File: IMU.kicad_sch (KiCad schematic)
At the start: 1 part, among them U2 4754

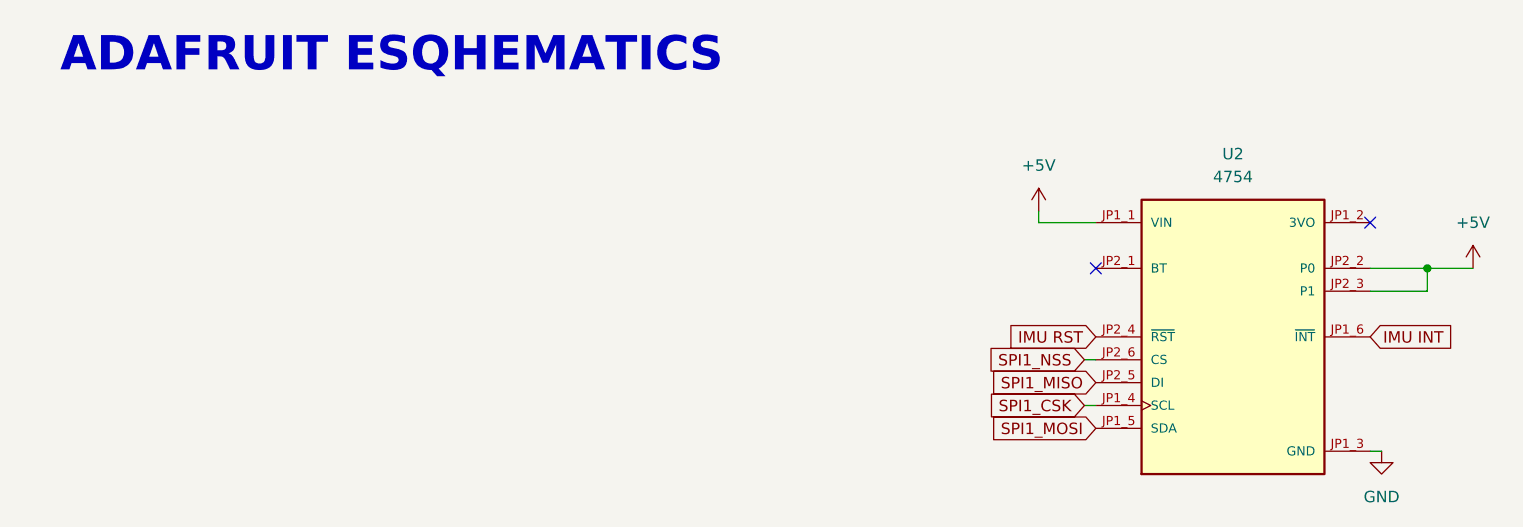
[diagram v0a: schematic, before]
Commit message: Todo antes de PCB
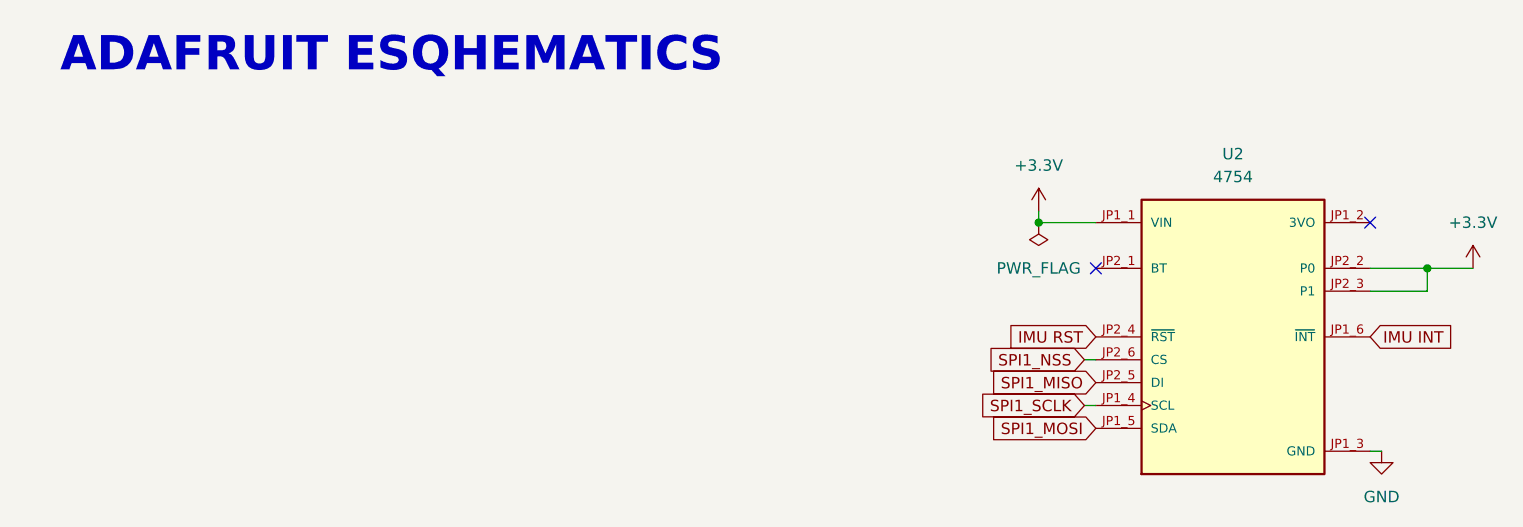
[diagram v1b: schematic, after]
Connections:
- net +5V renamed +3.3V
- net SPI1_CSK renamed SPI1_SCLK
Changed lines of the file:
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@@
 		(color 0 0 0 0)
 	)
+	(junction
+		(at 143.51 95.25)
+		(diameter 0)
+		(color 0 0 0 0)
+	)
 	(no_connect
 		(at 180.34 95.25)
@@
 		)
 	)
-	(global_label "SPI1_CSK"
+	(global_label "SPI1_SCLK"
 		(shape input)
 		(at 148.59 115.57 180)
@@
 		)
 		(property "Intersheetrefs" "${INTERSHEET_REFS}"
-			(at 136.5939 115.57 0)
+			(at 135.5658 115.57 0)
 			(hide yes)
 			(show_name no)
@@
 	)
 	(symbol
-		(lib_id "power:+5V")
-		(at 143.51 93.98 0)
-		(unit 1)
-		(body_style 1)
-		(exclude_from_sim no)
-		(in_bom yes)
-		(on_board yes)
-		(in_pos_files yes)
-		(dnp no)
-		(fields_autoplaced yes)
-		(property "Reference" "#PWR028"
-			(at 143.51 97.79 0)
-			(hide yes)
-			(show_name no)
-			(do_not_autoplace no)
-			(effects
-				(font
-					(size 1.27 1.27)
-				)
-			)
-		)
-		(property "Value" "+5V"
-			(at 143.51 88.9 0)
-			(show_name no)
-			(do_not_autoplace no)
-			(effects
-				(font
-					(size 1.27 1.27)
-				)
-			)
-		)
-		(property "Footprint" ""
-			(at 143.51 93.98 0)
-			(hide yes)
-			(show_name no)
-			(do_not_autoplace no)
-			(effects
-				(font
-					(size 1.27 1.27)
-				)
-			)
-		)
-		(property "Datasheet" ""
-			(at 143.51 93.98 0)
-			(hide yes)
-			(show_name no)
-			(do_not_autoplace no)
-			(effects
-				(font
-					(size 1.27 1.27)
-				)
-			)
-		)
-		(property "Description" "Power symbol creates a global label with name \"+5V\""
-			(at 143.51 93.98 0)
-			(hide yes)
-			(show_name no)
-			(do_not_autoplace no)
-			(effects
-				(font
-					(size 1.27 1.27)
-				)
-			)
-		)
-		(pin "1"
-		)
-		(instances
-			(project "ARLISS_STM32_2026"
-				(path "/9719ea46-14c4-4409-9c57-49dd5454c03f/243e1b39-32df-463e-8f3d-bc06fe39ea80"
-					(reference "#PWR028")
-					(unit 1)
-				)
-			)
-		)
-	)
-	(symbol
 		(lib_id "4754:4754")
 		(at 165.1 107.95 0)
@@
 			(at 165.1 107.95 0)
 			(hide yes)
-			(show_name no)
+			(show_name yes)
 			(do_not_autoplace no)
 			(effects
@@
 	)
 	(symbol
-		(lib_id "power:+5V")
+		(lib_id "power:+3.3V")
+		(at 143.51 93.98 0)
+		(unit 1)
+		(body_style 1)
+		(exclude_from_sim no)
+		(in_bom yes)
+		(on_board yes)
+		(in_pos_files yes)
+		(dnp no)
+		(fields_autoplaced yes)
+		(property "Reference" "#PWR028"
+			(at 143.51 97.79 0)
+			(hide yes)
+			(show_name no)
+			(do_not_autoplace no)
+			(effects
+				(font
+					(size 1.27 1.27)
+				)
+			)
+		)
+		(property "Value" "+3.3V"
+			(at 143.51 88.9 0)
+			(show_name no)
+			(do_not_autoplace no)
+			(effects
+				(font
+					(size 1.27 1.27)
+				)
+			)
+		)
+		(property "Footprint" ""
+			(at 143.51 93.98 0)
+			(hide yes)
+			(show_name no)
+			(do_not_autoplace no)
+			(effects
+				(font
+					(size 1.27 1.27)
+				)
+			)
+		)
+		(property "Datasheet" ""
+			(at 143.51 93.98 0)
+			(hide yes)
+			(show_name no)
+			(do_not_autoplace no)
+			(effects
+				(font
+					(size 1.27 1.27)
+				)
+			)
+		)
+		(property "Description" "Power symbol creates a global label with name \"+3.3V\""
+			(at 143.51 93.98 0)
+			(hide yes)
+			(show_name no)
+			(do_not_autoplace no)
+			(effects
+				(font
+					(size 1.27 1.27)
+				)
+			)
+		)
+		(pin "1"
+		)
+		(instances
+			(project "ARLISS_STM32_2026"
+				(path "/9719ea46-14c4-4409-9c57-49dd5454c03f/243e1b39-32df-463e-8f3d-bc06fe39ea80"
+					(reference "#PWR028")
+					(unit 1)
+				)
+			)
+		)
+	)
+	(symbol
+		(lib_id "power:PWR_FLAG")
+		(at 143.51 95.25 180)
+		(unit 1)
+		(body_style 1)
+		(exclude_from_sim no)
+		(in_bom yes)
+		(on_board yes)
+		(in_pos_files yes)
+		(dnp no)
+		(fields_autoplaced yes)
+		(property "Reference" "#FLG01"
+			(at 143.51 97.155 0)
+			(hide yes)
+			(show_name no)
+			(do_not_autoplace no)
+			(effects
+				(font
+					(size 1.27 1.27)
+				)
+			)
+		)
+		(property "Value" "PWR_FLAG"
+			(at 143.51 100.33 0)
+			(show_name no)
+			(do_not_autoplace no)
+			(effects
+				(font
+					(size 1.27 1.27)
+				)
+			)
+		)
+		(property "Footprint" ""
+			(at 143.51 95.25 0)
+			(hide yes)
+			(show_name no)
+			(do_not_autoplace no)
+			(effects
+				(font
+					(size 1.27 1.27)
+				)
+			)
+		)
+		(property "Datasheet" ""
+			(at 143.51 95.25 0)
+			(hide yes)
+			(show_name no)
+			(do_not_autoplace no)
+			(effects
+				(font
+					(size 1.27 1.27)
+				)
+			)
+		)
+		(property "Description" "Special symbol for telling ERC where power comes from"
+			(at 143.51 95.25 0)
+			(hide yes)
+			(show_name no)
+			(do_not_autoplace no)
+			(effects
+				(font
+					(size 1.27 1.27)
+				)
+			)
+		)
+		(pin "1"
+		)
+		(instances
+			(project "ARLISS_STM32_2026"
+				(path "/9719ea46-14c4-4409-9c57-49dd5454c03f/243e1b39-32df-463e-8f3d-bc06fe39ea80"
+					(reference "#FLG01")
+					(unit 1)
+				)
+			)
+		)
+	)
+	(symbol
+		(lib_id "power:+3.3V")
 		(at 191.77 100.33 0)
 		(unit 1)
@@
 			)
 		)
-		(property "Value" "+5V"
+		(property "Value" "+3.3V"
 			(at 191.77 95.25 0)
 			(show_name no)
@@
 			)
 		)
-		(property "Description" "Power symbol creates a global label with name \"+5V\""
+		(property "Description" "Power symbol creates a global label with name \"+3.3V\""
 			(at 191.77 100.33 0)
 			(hide yes)
